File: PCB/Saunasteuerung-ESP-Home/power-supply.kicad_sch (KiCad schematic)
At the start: 6 parts, among them J8 696106003002

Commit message: Added AD5593
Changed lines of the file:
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@@
 (kicad_sch
-	(version 20231120)
+	(version 20250114)
 	(generator "eeschema")
-	(generator_version "8.0")
+	(generator_version "9.0")
 	(paper "A4")
 	(junction

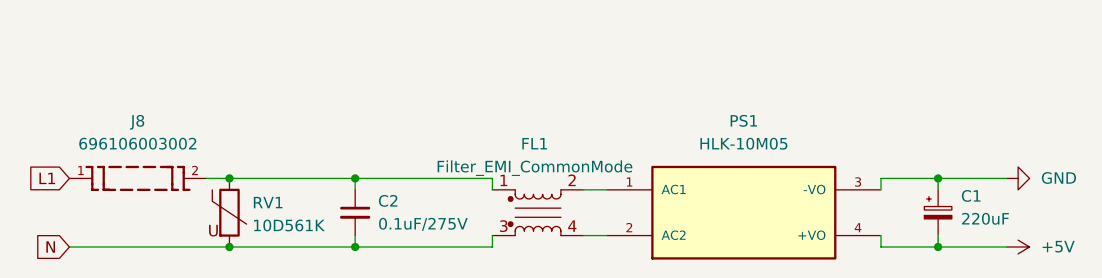
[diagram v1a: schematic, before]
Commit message: V2.0 push
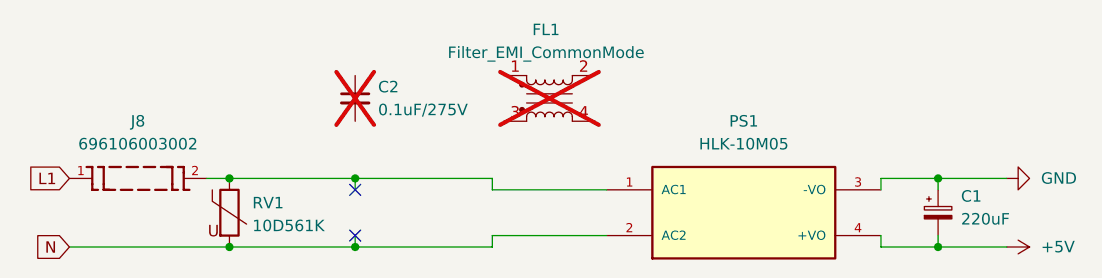
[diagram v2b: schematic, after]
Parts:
- C2, FL1: now not fitted; now left out of the parts list
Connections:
- net N: now also PS1.2 (AC2); no longer C2.2, FL1.3
- net at J8.2, RV1.1: now also PS1.1 (AC1); no longer C2.1, FL1.1
- net at FL1.2: no longer PS1.1 (AC1)
- net at FL1.4: no longer PS1.2 (AC2)
- no-connect marks 0 -> 2
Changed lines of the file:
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@@
 		(color 0 0 0 0)
 	)
+	(no_connect
+		(at 114.3 43.18)
+	)
+	(no_connect
+		(at 114.3 48.26)
+	)
+	(wire
+		(pts
+			(xy 129.54 43.18) (xy 142.24 43.18)
+		)
+		(stroke
+			(width 0)
+			(type default)
+		)
+	)
 	(wire
 		(pts
@@
 	(wire
 		(pts
-			(xy 139.7 48.26) (xy 142.24 48.26)
-		)
-		(stroke
-			(width 0)
-			(type default)
-		)
-	)
-	(wire
-		(pts
 			(xy 179.07 41.91) (xy 179.07 43.18)
 		)
@@
 	(wire
 		(pts
-			(xy 139.7 43.18) (xy 142.24 43.18)
-		)
-		(stroke
-			(width 0)
-			(type default)
-		)
-	)
-	(wire
-		(pts
 			(xy 100.33 41.91) (xy 114.3 41.91)
 		)
@@
 		(pts
 			(xy 100.33 49.53) (xy 114.3 49.53)
+		)
+		(stroke
+			(width 0)
+			(type default)
+		)
+	)
+	(wire
+		(pts
+			(xy 129.54 48.26) (xy 142.24 48.26)
 		)
 		(stroke
@@
 				(justify right)
 				(hide yes)
-			)
-		)
-	)
-	(symbol
-		(lib_id "Device:C_Small")
-		(at 114.3 45.72 0)
-		(unit 1)
-		(exclude_from_sim no)
-		(in_bom yes)
-		(on_board yes)
-		(dnp no)
-		(fields_autoplaced yes)
-		(property "Reference" "C2"
-			(at 116.84 44.4562 0)
-			(effects
-				(font
-					(size 1.27 1.27)
-				)
-				(justify left)
-			)
-		)
-		(property "Value" "0.1uF/275V"
-			(at 116.84 46.9962 0)
-			(effects
-				(font
-					(size 1.27 1.27)
-				)
-				(justify left)
-			)
-		)
-		(property "Footprint" ""
-			(at 114.3 45.72 0)
-			(effects
-				(font
-					(size 1.27 1.27)
-				)
-				(hide yes)
-			)
-		)
-		(property "Datasheet" "~"
-			(at 114.3 45.72 0)
-			(effects
-				(font
-					(size 1.27 1.27)
-				)
-				(hide yes)
-			)
-		)
-		(property "Description" "Unpolarized capacitor, small symbol"
-			(at 114.3 45.72 0)
-			(effects
-				(font
-					(size 1.27 1.27)
-				)
-				(hide yes)
-			)
-		)
-		(pin "2"
-		)
-		(pin "1"
-		)
-		(instances
-			(project "Saunasteuerung-ESP-Home"
-				(path "/c2709fca-2df2-4b64-83dc-e0d31f28d840/23bb9531-753a-4bf2-b6f9-22c6f38d7367"
-					(reference "C2")
-					(unit 1)
-				)
 			)
 		)
@@
 				)
 			)
+			(project "power-supply"
+				(path "/f6a42888-f9cb-481c-bc75-d972835775bc"
+					(reference "C2")
+					(unit 1)
+				)
+			)
 		)
 	)
@@
 				)
 			)
+			(project "power-supply"
+				(path "/f6a42888-f9cb-481c-bc75-d972835775bc"
+					(reference "#PWR02")
+					(unit 1)
+				)
+			)
 		)
 	)
@@
 				)
 			)
+			(project "power-supply"
+				(path "/f6a42888-f9cb-481c-bc75-d972835775bc"
+					(reference "#PWR01")
+					(unit 1)
+				)
+			)
 		)
 	)
@@
 				)
 			)
+			(project "power-supply"
+				(path "/f6a42888-f9cb-481c-bc75-d972835775bc"
+					(reference "PS1")
+					(unit 1)
+				)
+			)
 		)
 	)
 	(symbol
 		(lib_id "Device:Filter_EMI_CommonMode")
-		(at 134.62 45.72 0)
+		(at 135.89 33.02 0)
 		(unit 1)
 		(exclude_from_sim no)
-		(in_bom yes)
-		(on_board yes)
-		(dnp no)
+		(in_bom no)
+		(on_board no)
+		(dnp yes)
 		(fields_autoplaced yes)
 		(property "Reference" "FL1"
-			(at 134.239 38.1 0)
+			(at 135.509 25.4 0)
 			(effects
 				(font
@@
 		)
 		(property "Value" "Filter_EMI_CommonMode"
-			(at 134.239 40.64 0)
+			(at 135.509 27.94 0)
 			(effects
 				(font
@@
 		)
 		(property "Footprint" "Inductor_THT:L_CommonMode_PulseElectronics_PH9455x105NL_1"
-			(at 134.62 44.704 0)
+			(at 135.89 32.004 0)
 			(effects
 				(font
@@
 		)
 		(property "Datasheet" "~"
-			(at 134.62 44.704 0)
+			(at 135.89 32.004 0)
 			(effects
 				(font
@@
 		)
 		(property "Description" "EMI 2-inductor common mode filter"
-			(at 134.62 45.72 0)
+			(at 135.89 33.02 0)
 			(effects
 				(font
@@
 				)
 			)
+			(project "power-supply"
+				(path "/f6a42888-f9cb-481c-bc75-d972835775bc"
+					(reference "RV1")
+					(unit 1)
+				)
+			)
+		)
+	)
+	(symbol
+		(lib_id "Device:C_Small")
+		(at 114.3 33.02 0)
+		(unit 1)
+		(exclude_from_sim no)
+		(in_bom no)
+		(on_board no)
+		(dnp yes)
+		(fields_autoplaced yes)
+		(property "Reference" "C2"
+			(at 116.84 31.7562 0)
+			(effects
+				(font
+					(size 1.27 1.27)
+				)
+				(justify left)
+			)
+		)
+		(property "Value" "0.1uF/275V"
+			(at 116.84 34.2962 0)
+			(effects
+				(font
+					(size 1.27 1.27)
+				)
+				(justify left)
+			)
+		)
+		(property "Footprint" ""
+			(at 114.3 33.02 0)
+			(effects
+				(font
+					(size 1.27 1.27)
+				)
+				(hide yes)
+			)
+		)
+		(property "Datasheet" "~"
+			(at 114.3 33.02 0)
+			(effects
+				(font
+					(size 1.27 1.27)
+				)
+				(hide yes)
+			)
+		)
+		(property "Description" "Unpolarized capacitor, small symbol"
+			(at 114.3 33.02 0)
+			(effects
+				(font
+					(size 1.27 1.27)
+				)
+				(hide yes)
+			)
+		)
+		(pin "2"
+		)
+		(pin "1"
+		)
+		(instances
+			(project "Saunasteuerung-ESP-Home"
+				(path "/c2709fca-2df2-4b64-83dc-e0d31f28d840/23bb9531-753a-4bf2-b6f9-22c6f38d7367"
+					(reference "C2")
+					(unit 1)
+				)
+			)
 		)
 	)
@@
 				)
 			)
-		)
-	)
+			(project "power-supply"
+				(path "/f6a42888-f9cb-481c-bc75-d972835775bc"
+					(reference "J1")
+					(unit 1)
+				)
+			)
+		)
+	)
+	(sheet_instances
+		(path "/"
+			(page "1")
+		)
+	)
+	(embedded_fonts no)
 )
